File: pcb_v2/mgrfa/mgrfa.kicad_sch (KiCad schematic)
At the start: 50 parts, among them J8 bus_mgrf_1, J9 bus_mgrf_2, U1 74LS574, U2 74LS574, U3 74LS574, U4 74LS574, U5 74LS574, U6 74LS574, U7 74LS574, U8 74LS138, U9 74HC238

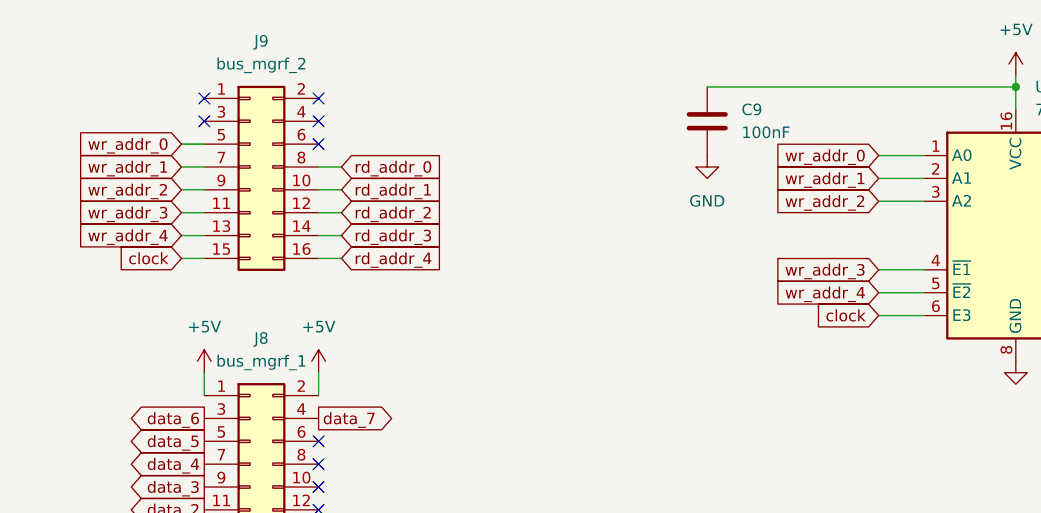
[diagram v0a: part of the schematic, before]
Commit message: Update mgrfa.kicad_pcb and mgrfa.kicad_sch
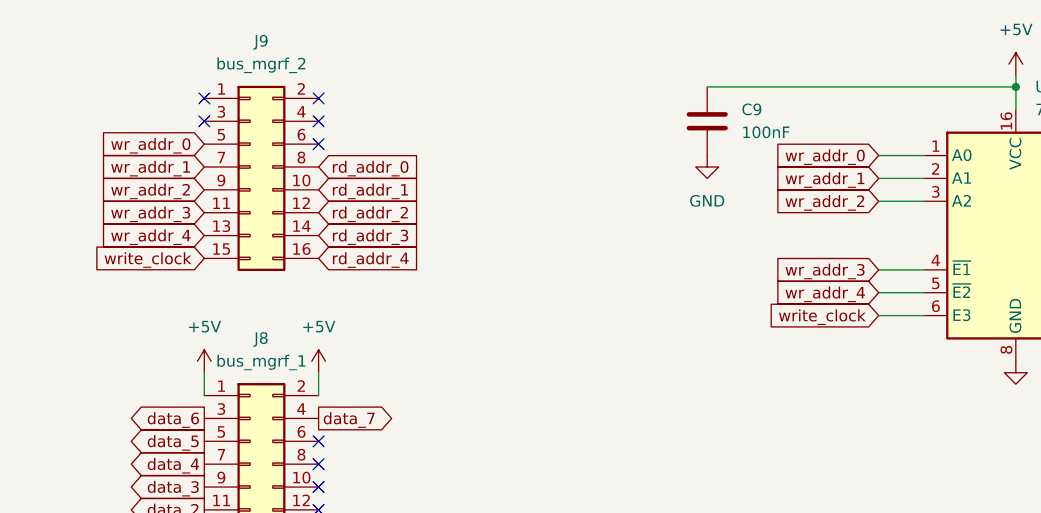
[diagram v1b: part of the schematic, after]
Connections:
- net clock renamed write_clock
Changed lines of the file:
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@@
 	)
 	(no_connect
-		(at 45.72 22.86)
-	)
-	(no_connect
 		(at 33.02 25.4)
 	)
@@
 		(at 133.35 29.21)
 	)
+	(no_connect
+		(at 45.72 22.86)
+	)
 	(wire
 		(pts
@@
 	(wire
 		(pts
-			(xy 48.26 38.1) (xy 45.72 38.1)
-		)
-		(stroke
-			(width 0)
-			(type default)
-		)
-	)
-	(wire
-		(pts
-			(xy 30.48 35.56) (xy 33.02 35.56)
-		)
-		(stroke
-			(width 0)
-			(type default)
-		)
-	)
-	(wire
-		(pts
 			(xy 73.66 184.15) (xy 77.47 184.15)
 		)
@@
 	(wire
 		(pts
-			(xy 48.26 40.64) (xy 45.72 40.64)
-		)
-		(stroke
-			(width 0)
-			(type default)
-		)
-	)
-	(wire
-		(pts
 			(xy 173.99 46.99) (xy 176.53 46.99)
 		)
@@
 	(wire
 		(pts
-			(xy 48.26 35.56) (xy 45.72 35.56)
-		)
-		(stroke
-			(width 0)
-			(type default)
-		)
-	)
-	(wire
-		(pts
 			(xy 328.93 171.45) (xy 332.74 171.45)
 		)
@@
 	(wire
 		(pts
-			(xy 30.48 33.02) (xy 33.02 33.02)
-		)
-		(stroke
-			(width 0)
-			(type default)
-		)
-	)
-	(wire
-		(pts
 			(xy 205.74 36.83) (xy 201.93 36.83)
 		)
@@
 	(wire
 		(pts
-			(xy 30.48 27.94) (xy 33.02 27.94)
-		)
-		(stroke
-			(width 0)
-			(type default)
-		)
-	)
-	(wire
-		(pts
 			(xy 138.43 171.45) (xy 140.97 171.45)
 		)
@@
 	(wire
 		(pts
-			(xy 30.48 30.48) (xy 33.02 30.48)
-		)
-		(stroke
-			(width 0)
-			(type default)
-		)
-	)
-	(wire
-		(pts
 			(xy 238.76 153.67) (xy 238.76 151.13)
 		)
@@
 	(wire
 		(pts
-			(xy 48.26 33.02) (xy 45.72 33.02)
-		)
-		(stroke
-			(width 0)
-			(type default)
-		)
-	)
-	(wire
-		(pts
 			(xy 346.71 184.15) (xy 353.06 184.15)
 		)
@@
 	(wire
 		(pts
-			(xy 30.48 40.64) (xy 33.02 40.64)
-		)
-		(stroke
-			(width 0)
-			(type default)
-		)
-	)
-	(wire
-		(pts
 			(xy 340.36 171.45) (xy 342.9 171.45)
 		)
@@
 	(wire
 		(pts
-			(xy 48.26 30.48) (xy 45.72 30.48)
-		)
-		(stroke
-			(width 0)
-			(type default)
-		)
-	)
-	(wire
-		(pts
 			(xy 175.26 41.91) (xy 175.26 21.59)
 		)
@@
 	(wire
 		(pts
-			(xy 30.48 38.1) (xy 33.02 38.1)
-		)
-		(stroke
-			(width 0)
-			(type default)
-		)
-	)
-	(wire
-		(pts
 			(xy 44.45 184.15) (xy 50.8 184.15)
 		)
@@
 	(global_label "rd_addr_1"
 		(shape input)
-		(at 48.26 33.02 0)
+		(at 45.72 33.02 0)
 		(fields_autoplaced yes)
 		(effects
@@
 		)
 		(property "Intersheetrefs" "${INTERSHEET_REFS}"
-			(at 59.9864 32.9406 0)
+			(at 57.4464 32.9406 0)
 			(effects
 				(font
@@
 	(global_label "rd_addr_2"
 		(shape input)
-		(at 48.26 35.56 0)
+		(at 45.72 35.56 0)
 		(fields_autoplaced yes)
 		(effects
@@
 		)
 		(property "Intersheetrefs" "${INTERSHEET_REFS}"
-			(at 59.9864 35.4806 0)
+			(at 57.4464 35.4806 0)
 			(effects
 				(font
@@
 		)
 	)
-	(global_label "clock"
+	(global_label "write_clock"
 		(shape input)
 		(at 107.95 46.99 180)
@@
 		)
 		(property "Intersheetrefs" "${INTERSHEET_REFS}"
-			(at 99.9453 46.99 0)
+			(at 94.4419 46.99 0)
 			(effects
 				(font
@@
 	(global_label "wr_addr_0"
 		(shape input)
-		(at 30.48 27.94 180)
+		(at 33.02 27.94 180)
 		(fields_autoplaced yes)
 		(effects
@@
 		)
 		(property "Intersheetrefs" "${INTERSHEET_REFS}"
-			(at 18.5721 27.8606 0)
+			(at 21.1121 27.8606 0)
 			(effects
 				(font
@@
 	(global_label "wr_addr_4"
 		(shape input)
-		(at 30.48 38.1 180)
+		(at 33.02 38.1 180)
 		(fields_autoplaced yes)
 		(effects
@@
 		)
 		(property "Intersheetrefs" "${INTERSHEET_REFS}"
-			(at 18.5721 38.0206 0)
+			(at 21.1121 38.0206 0)
 			(effects
 				(font
@@
 	(global_label "rd_addr_3"
 		(shape input)
-		(at 48.26 38.1 0)
+		(at 45.72 38.1 0)
 		(fields_autoplaced yes)
 		(effects
@@
 		)
 		(property "Intersheetrefs" "${INTERSHEET_REFS}"
-			(at 59.9864 38.0206 0)
+			(at 57.4464 38.0206 0)
 			(effects
 				(font
@@
 		)
 	)
-	(global_label "clock"
+	(global_label "write_clock"
 		(shape input)
-		(at 30.48 40.64 180)
+		(at 33.02 40.64 180)
 		(fields_autoplaced yes)
 		(effects
@@
 		)
 		(property "Intersheetrefs" "${INTERSHEET_REFS}"
-			(at 23.0474 40.7194 0)
+			(at 19.5119 40.64 0)
 			(effects
 				(font
@@
 	(global_label "wr_addr_1"
 		(shape input)
-		(at 30.48 30.48 180)
+		(at 33.02 30.48 180)
 		(fields_autoplaced yes)
 		(effects
@@
 		)
 		(property "Intersheetrefs" "${INTERSHEET_REFS}"
-			(at 18.5721 30.4006 0)
+			(at 21.1121 30.4006 0)
 			(effects
 				(font
@@
 	(global_label "wr_addr_2"
 		(shape input)
-		(at 30.48 33.02 180)
+		(at 33.02 33.02 180)
 		(fields_autoplaced yes)
 		(effects
@@
 		)
 		(property "Intersheetrefs" "${INTERSHEET_REFS}"
-			(at 18.5721 32.9406 0)
+			(at 21.1121 32.9406 0)
 			(effects
 				(font
@@
 	(global_label "rd_addr_4"
 		(shape input)
-		(at 48.26 40.64 0)
+		(at 45.72 40.64 0)
 		(fields_autoplaced yes)
 		(effects
@@
 		)
 		(property "Intersheetrefs" "${INTERSHEET_REFS}"
-			(at 59.9864 40.5606 0)
+			(at 57.4464 40.5606 0)
 			(effects
 				(font
@@
 	(global_label "wr_addr_3"
 		(shape input)
-		(at 30.48 35.56 180)
+		(at 33.02 35.56 180)
 		(fields_autoplaced yes)
 		(effects
@@
 		)
 		(property "Intersheetrefs" "${INTERSHEET_REFS}"
-			(at 18.5721 35.4806 0)
+			(at 21.1121 35.4806 0)
 			(effects
 				(font
@@
 	(global_label "rd_addr_0"
 		(shape input)
-		(at 48.26 30.48 0)
+		(at 45.72 30.48 0)
 		(fields_autoplaced yes)
 		(effects
@@
 		)
 		(property "Intersheetrefs" "${INTERSHEET_REFS}"
-			(at 59.9864 30.4006 0)
+			(at 57.4464 30.4006 0)
 			(effects
 				(font
